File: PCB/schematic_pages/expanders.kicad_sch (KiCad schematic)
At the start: 32 parts

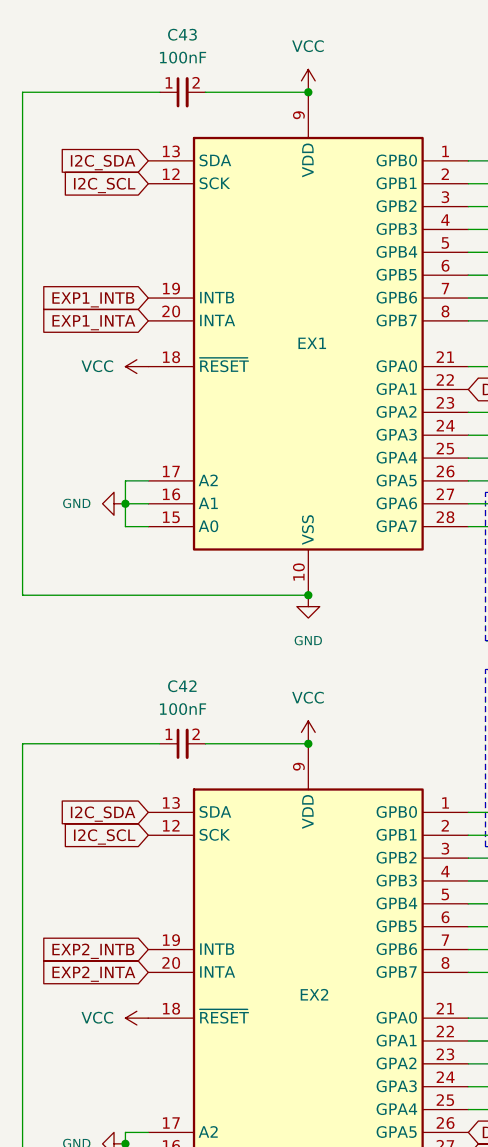
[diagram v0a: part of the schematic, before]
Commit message: repo rearrange
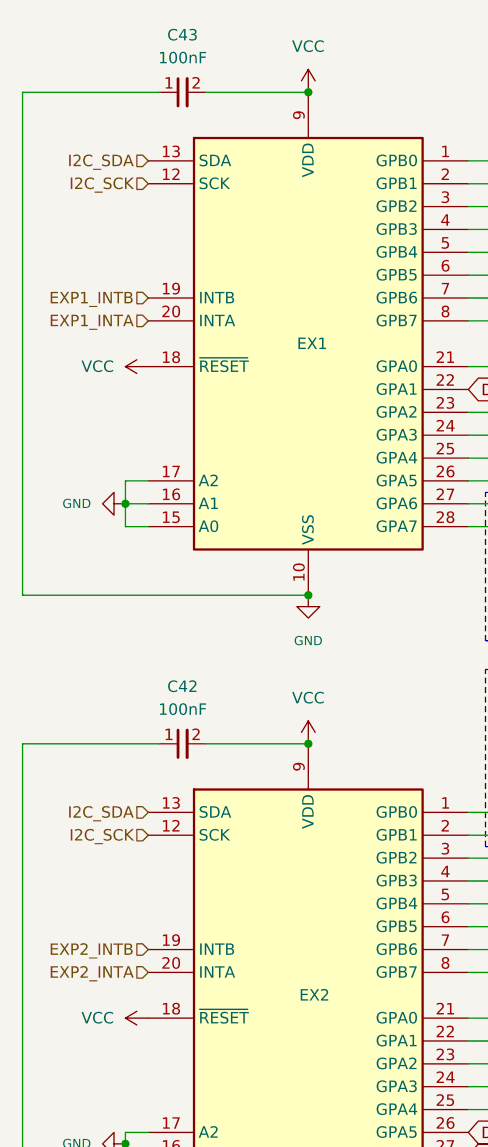
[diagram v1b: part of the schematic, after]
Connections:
- net I2C_SCL renamed I2C_SCK
